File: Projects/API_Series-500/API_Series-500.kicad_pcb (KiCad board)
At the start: 2 copper layers, 152.3 x 105 mm, 1 part, among them J1 EDA 306

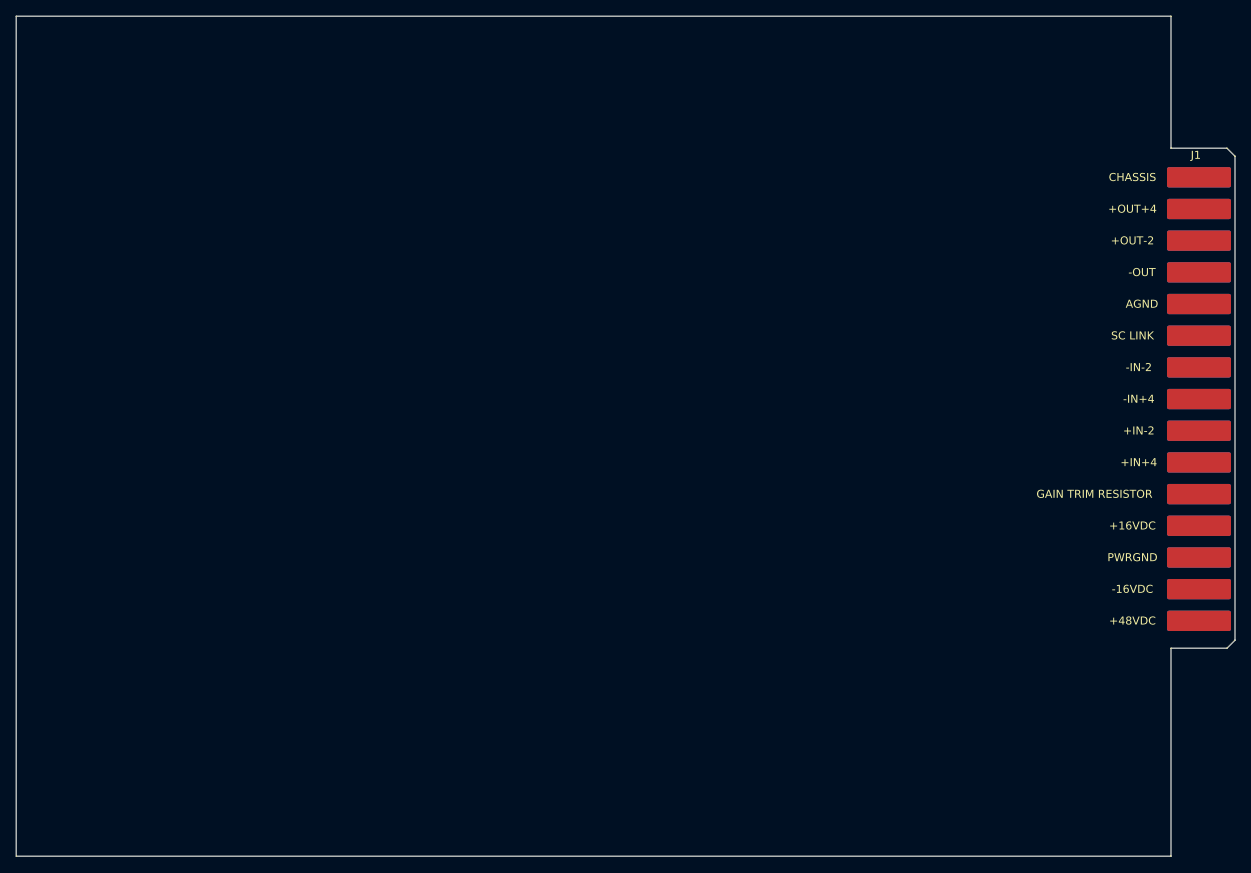
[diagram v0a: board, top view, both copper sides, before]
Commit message: adding parts placer position file to api 500
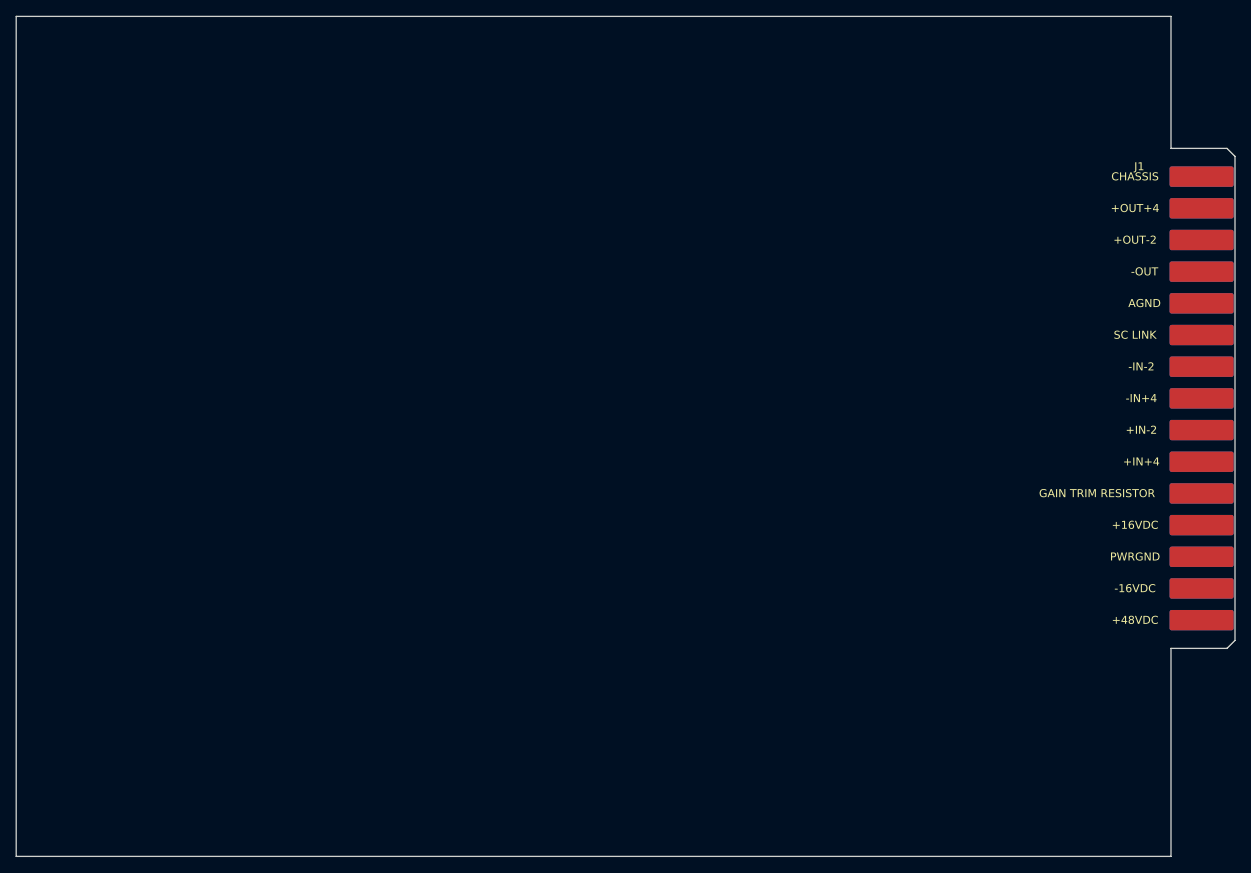
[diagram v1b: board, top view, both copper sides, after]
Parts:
- added BOARD: board, Library:board, F.Cu at (126.8, 107.5)
- moved J1 3.89 mm to (198.8, 102.8)
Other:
- board text removed: "Cut here in case mounted on "L" shaped Aluminium support leaving room for screws form the front panel"
- board text removed: "Cut here in case mounted on "L" shaped aluminium support directly in physical contact with the PCB"
- board text removed: "No room between the PCB and the front panel"
